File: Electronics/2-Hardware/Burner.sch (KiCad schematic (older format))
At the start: 19 parts, among them P1 CONN_2, P2 CONN_2, P3 CONN_1, P5 CONN_2, P6 CONN_1, Q1 DMN2230U-7, U2 MSP430G2553-20, U3 ISL32612

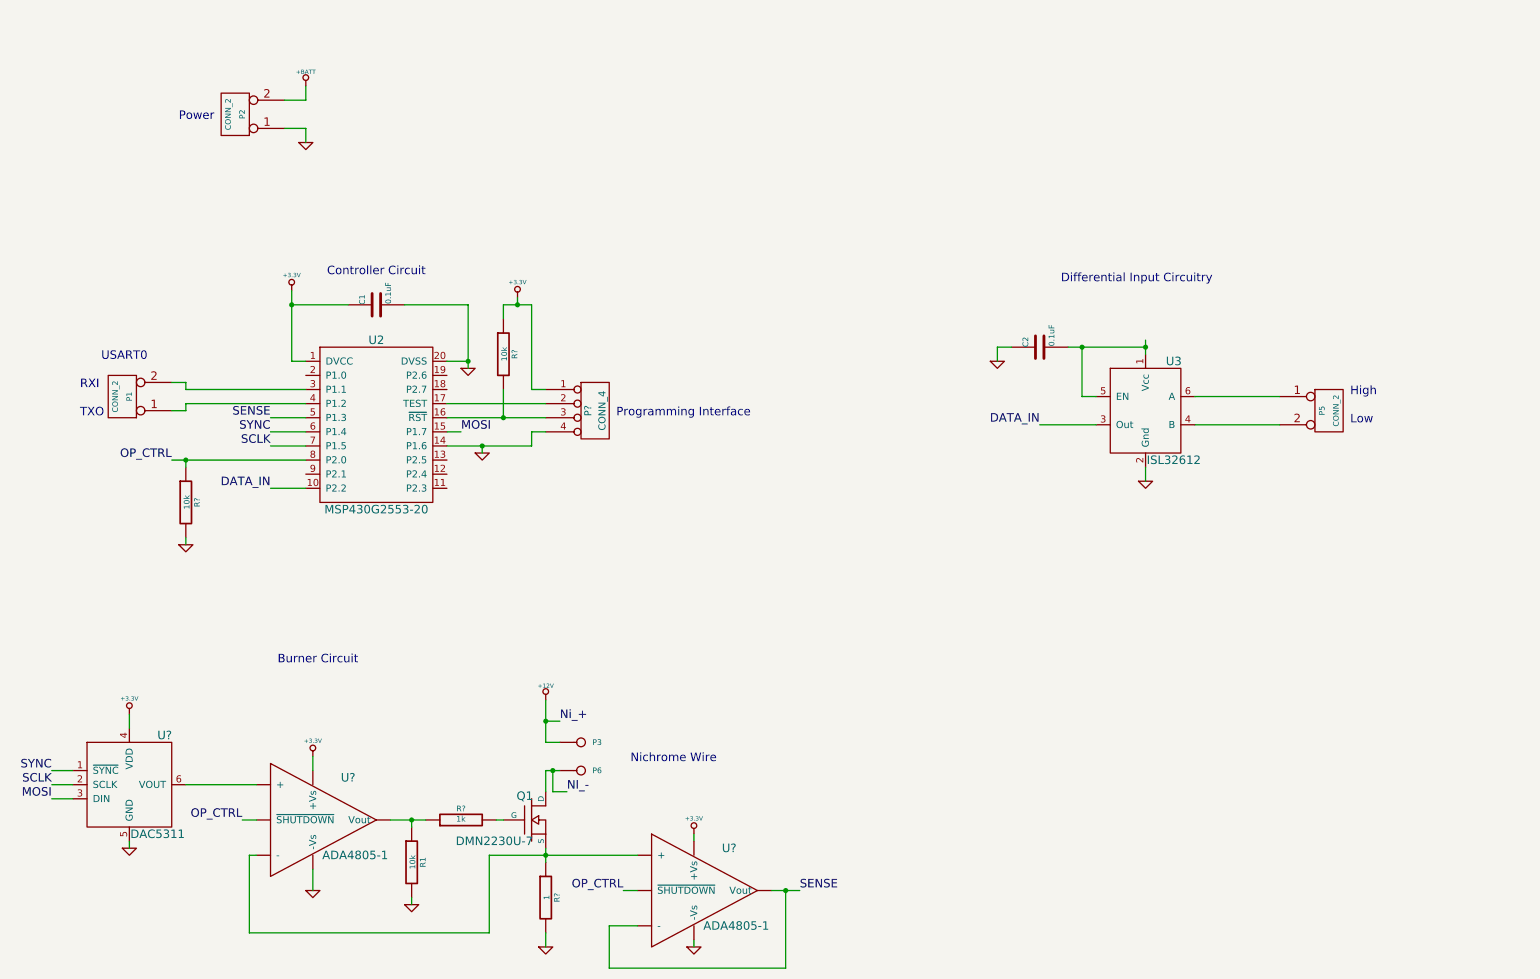
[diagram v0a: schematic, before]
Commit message: Added boost convertor to schematic
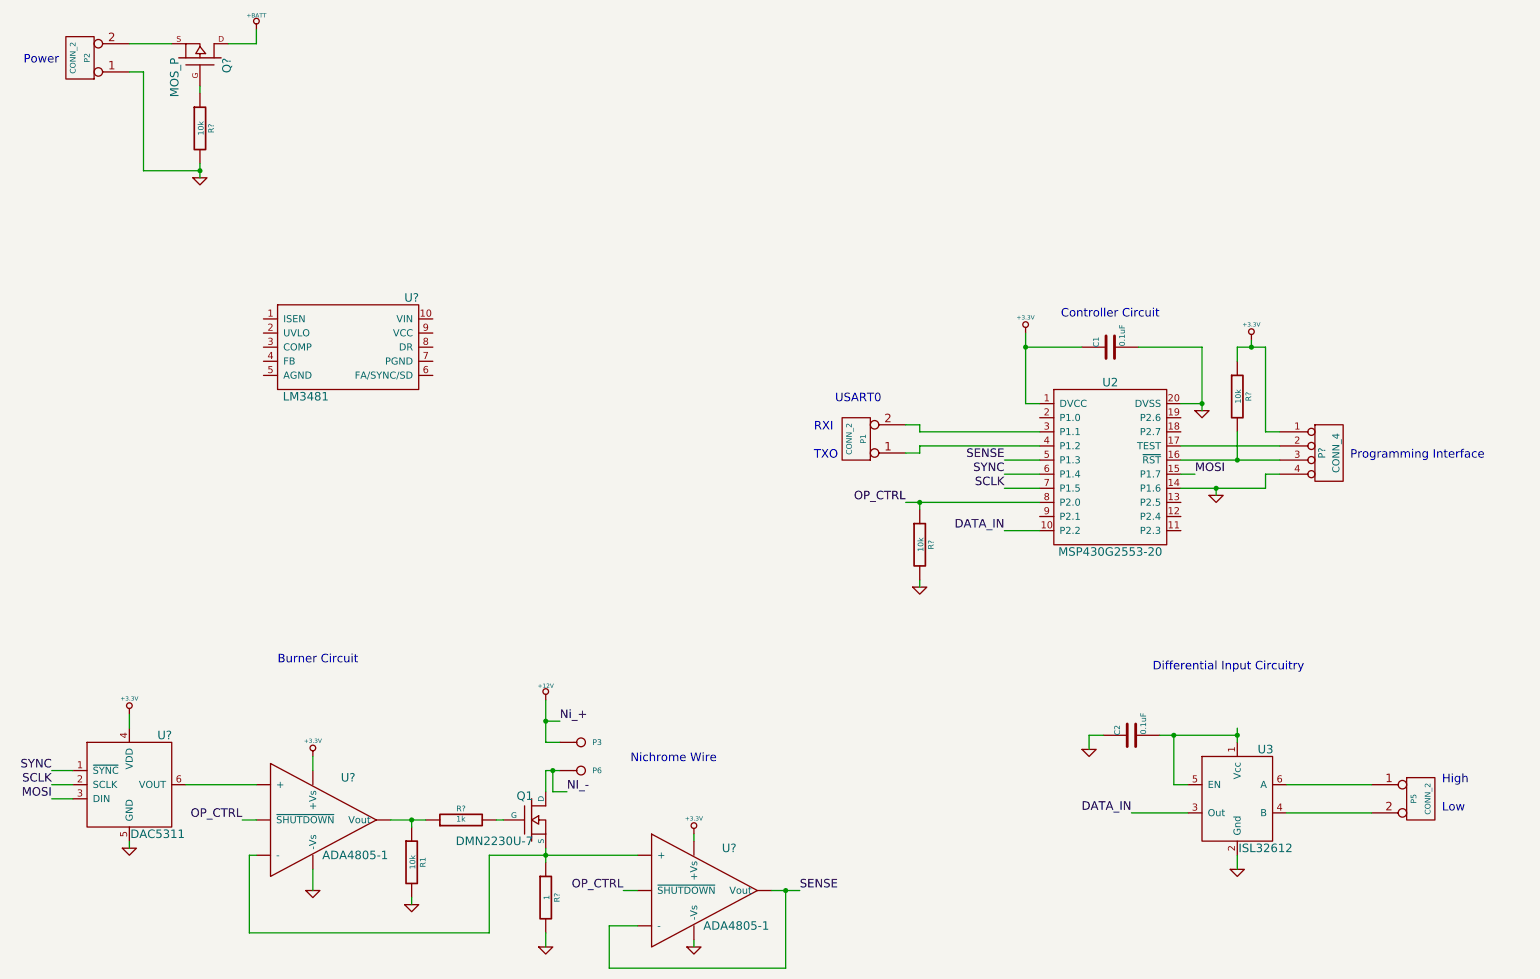
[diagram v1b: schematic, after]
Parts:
- added Q?: MOS_P, ~, symbol MOS_P
- added R?: 10k, ~, symbol R
- added U?: LM3481, symbol LM3481
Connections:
- net +BATT: now also Q?.D; no longer P2.2 (PM)
- net GND: now also R?.2
- new net: P2.2 (PM), Q?.S
- new net: Q?.G, R?.1
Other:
- moved on the sheet: C1, C2, P1, P2, P5, P?, R?, U2, U3
